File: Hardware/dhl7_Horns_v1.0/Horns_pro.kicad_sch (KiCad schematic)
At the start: 8 parts, among them J1 Conn_01x03, J2 Conn_01x02, J3 Conn_01x02, J4 Conn_01x02, Q1 Q_NMOS_DGS

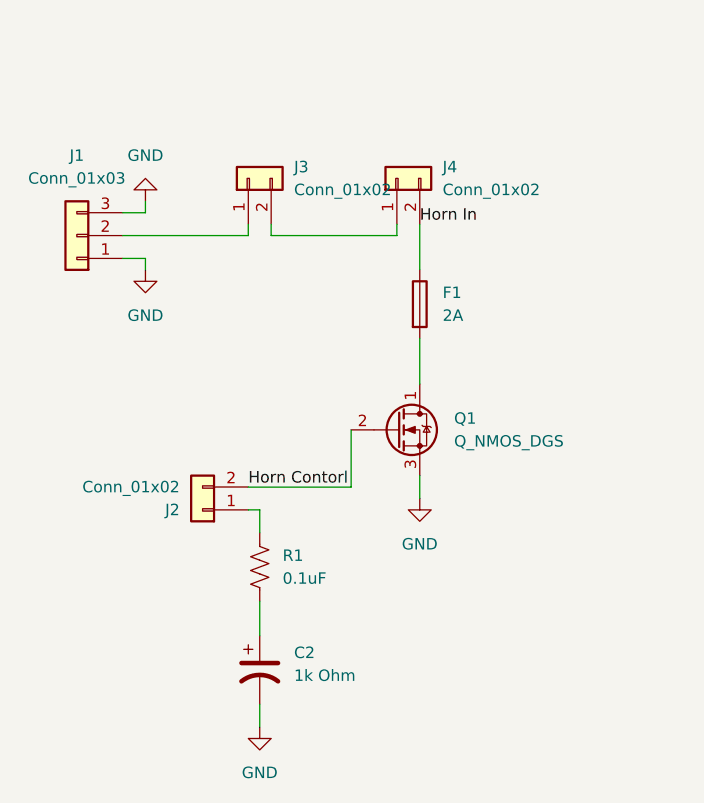
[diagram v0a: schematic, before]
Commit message: horns board
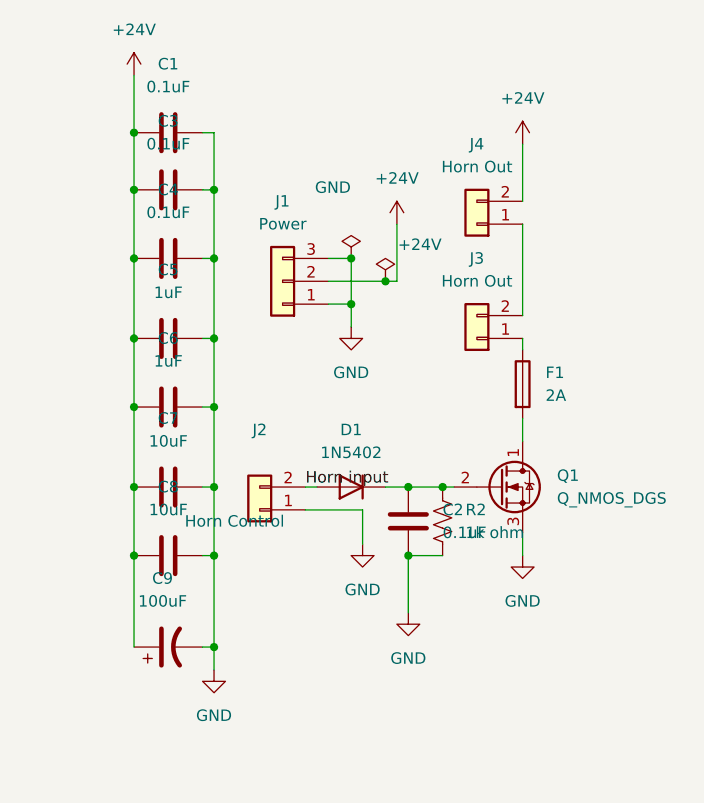
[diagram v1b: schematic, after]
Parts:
- removed R1: 0.1uF, symbol Device:R_US
- added C1, C3, C4: 0.1uF, Capacitor_SMD:C_0603_1608Metric_Pad1.08x0.95mm_HandSolder, symbol device:C
- added C5, C6: 1uF, Capacitor_SMD:C_0603_1608Metric_Pad1.08x0.95mm_HandSolder, symbol device:C
- added C7, C8: 10uF, Capacitor_SMD:C_0603_1608Metric_Pad1.08x0.95mm_HandSolder, symbol device:C
- added C9: 100uF, Capacitor_SMD:C_0603_1608Metric_Pad1.08x0.95mm_HandSolder, symbol Device:C_Polarized_US
- added D1: 1N5402, Diode_THT:D_DO-201AD_P15.24mm_Horizontal, symbol Diode:1N5402
- added R2: 1k ohm, Resistor_SMD:R_0603_1608Metric_Pad0.98x0.95mm_HandSolder, symbol Device:R_US
- C2: value 1k Ohm -> 0.1uF; footprint (none) -> Capacitor_SMD:C_0603_1608Metric_Pad1.08x0.95mm_HandSolder; symbol Device:C_Polarized_US -> device:C; MPN (none) -> 0201W104K100LE
- F1: footprint (none) -> Fuse:Fuse_1206_3216Metric; MPN (none) -> ERB-RD2R00X
- J1: value Conn_01x03 -> Power; footprint (none) -> Connector_Molex:Molex_KK-254_AE-6410-03A_1x03_P2.54mm_Vertical; MPN (none) -> 0022232031
- J2: value Conn_01x02 -> Horn Control; footprint (none) -> Connector_Molex:Molex_KK-254_AE-6410-02A_1x02_P2.54mm_Vertical; MPN (none) -> 0022232021
- J3, J4: value Conn_01x02 -> Horn Out; footprint (none) -> Connector_Molex:Molex_KK-254_AE-6410-02A_1x02_P2.54mm_Vertical; MPN (none) -> 0022232021
- Q1: footprint (none) -> Package_TO_SOT_SMD:TO-252-2; MPN (none) -> IRFR010PBF
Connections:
- net GND: now also C2.1, J2.1 (Pin_1), C1.2, C3.2, C4.2, C5.2, C6.2, C7.2, C8.2, C9.2, R2.1; no longer C2.2
- net at J3.1 (Pin_1): now also F1.1; no longer J1.2 (Pin_2)
- net Horn Contorl: no longer names the net of Q1.2 (G)
- net Horn Contorl: now also C2.2, D1.1 (K), R2.2; no longer J2.2 (Pin_2)
- net Horn In renamed +24V
- net +24V: now also J1.2 (Pin_2), C1.1, C3.1, C4.1, C5.1, C6.1, C7.1, C8.1, C9.1; no longer F1.1
- new net Horn input: D1.2 (A), J2.2 (Pin_2)
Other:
- moved on the sheet: F1, J1, J2, J3, J4, Q1
